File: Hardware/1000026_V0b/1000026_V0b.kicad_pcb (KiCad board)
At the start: 4 copper layers, 100 x 70 mm, 29 parts, among them J1 MOLEX_533750410, J2 4390, J3 532580229, J5 532580229, J9 0525591853, SW1 SW4_TL3305CF260QG_EWI, U1 TO252-3_ROM, U2 MAX7480ESA+

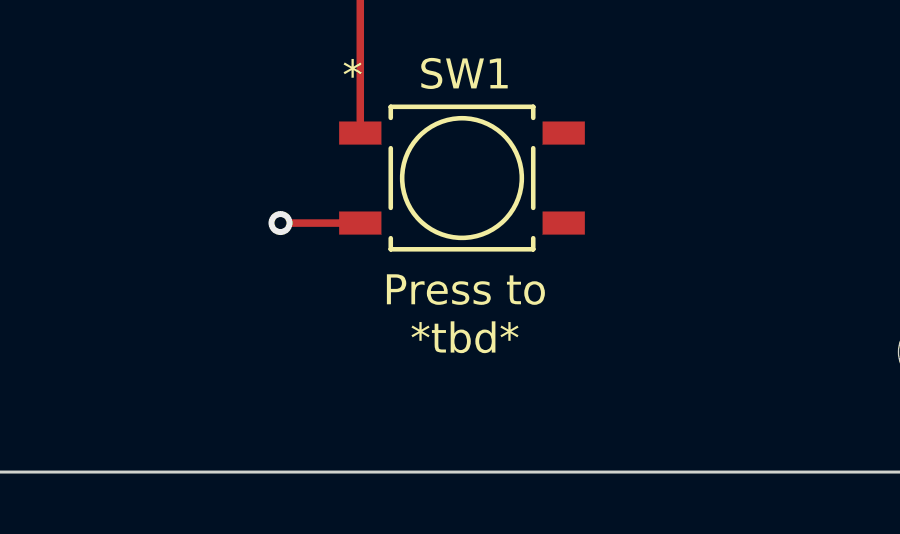
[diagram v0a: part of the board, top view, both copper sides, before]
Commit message: Updating PCB 1000026_V0a
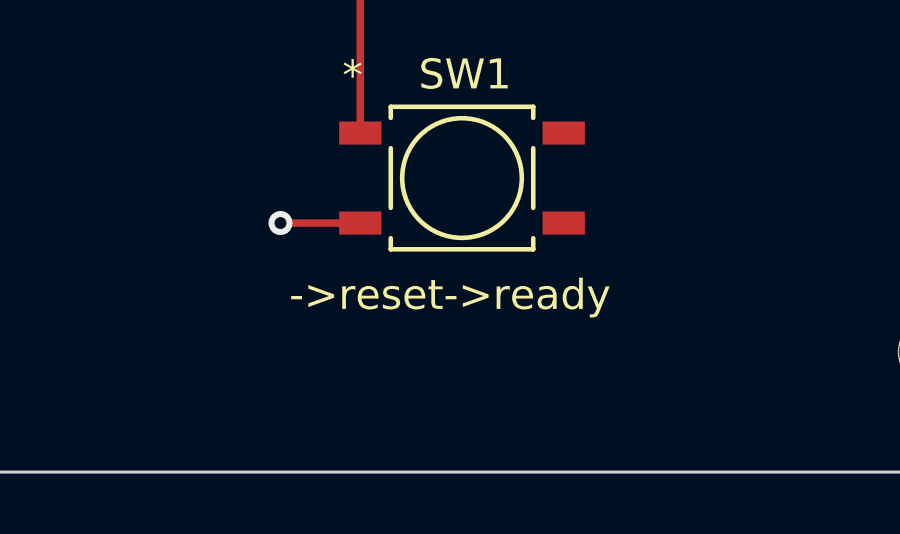
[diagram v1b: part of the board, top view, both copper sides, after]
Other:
- board text added: "->reset->ready"
- board text removed: "Press to *tbd*"
- board text removed: "Update {dblquote}tbd{dblquote} text"
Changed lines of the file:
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@@
     (effects (font (size 1 1) (thickness 0.2)))
   )
-  (gr_text "Press to \n*tbd*\n" (at 177.6898 117.9632) (layer "F.SilkS")
+  (gr_text "->reset->ready" (at 177.1898 117.3132) (layer "F.SilkS")
     (effects (font (size 1 1) (thickness 0.2)))
   )
@@
   )
   (gr_text "Center the ribbon\ncable connector.\n" (at 206.0148 87.5382) (layer "Cmts.User")
-    (effects (font (size 1 1) (thickness 0.2)))
-  )
-  (gr_text "Update {dblquote}tbd{dblquote} text" (at 178.1398 126.3632) (layer "Cmts.User")
     (effects (font (size 1 1) (thickness 0.2)))
   )
@@
     (height 19.825)
     (orientation 1)
-    (gr_text "70.0000 mm" (at 211.4198 88.2132 90) (layer "User.2")
+    (gr_text "70.0000 mm" (at 211.0898 88.2132 90) (layer "User.2")
       (effects (font (size 1 1) (thickness 0.2)))
     )
@@
     (height 13.208)
     (orientation 1)
-    (gr_text "62.0000 mm" (at 205.3608 88.2132 90) (layer "User.2")
+    (gr_text "62.0000 mm" (at 205.0308 88.2132 90) (layer "User.2")
       (effects (font (size 1 1) (thickness 0.2)))
     )
@@
     (height -11.366)
     (orientation 0)
-    (gr_text "92.0000 mm" (at 147.2398 44.9772) (layer "User.2")
+    (gr_text "92.0000 mm" (at 147.2398 44.6472) (layer "User.2")
       (effects (font (size 1 1) (thickness 0.2)))
     )
@@
     (height -14.7)
     (orientation 0)
-    (gr_text "100.0000 mm" (at 147.2398 42.4182) (layer "User.2")
+    (gr_text "100.0000 mm" (at 147.2398 42.0882) (layer "User.2")
       (effects (font (size 1 1) (thickness 0.2)))
     )
